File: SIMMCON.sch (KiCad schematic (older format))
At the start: 12 parts, among them U0 PALCE16V8H, U1 74AC(T)245, U2 74AC(T)245

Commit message: update some parts to soic
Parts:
- U1, U2: footprint Housings_DIP:DIP-20_W7.62mm -> Housings_SOIC:SOIC-20W_7.5x12.8mm_Pitch1.27mm
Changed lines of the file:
@@
 F 0 "U1" H 5250 2415 50  0000 C CNN
 F 1 "74AC(T)245" H 5250 2324 50  0000 C CNN
-F 2 "Housings_DIP:DIP-20_W7.62mm" H 5250 1700 50  0001 C CNN
+F 2 "Housings_SOIC:SOIC-20W_7.5x12.8mm_Pitch1.27mm" H 5250 1700 50  0001 C CNN
 F 3 "" H 5250 1700 50  0001 C CNN
 	1    5250 1700
@@
 F 0 "U2" H 5250 3815 50  0000 C CNN
 F 1 "74AC(T)245" H 5250 3724 50  0000 C CNN
-F 2 "Housings_DIP:DIP-20_W7.62mm" H 5250 3100 50  0001 C CNN
+F 2 "Housings_SOIC:SOIC-20W_7.5x12.8mm_Pitch1.27mm" H 5250 3100 50  0001 C CNN
 F 3 "" H 5250 3100 50  0001 C CNN
 	1    5250 3100

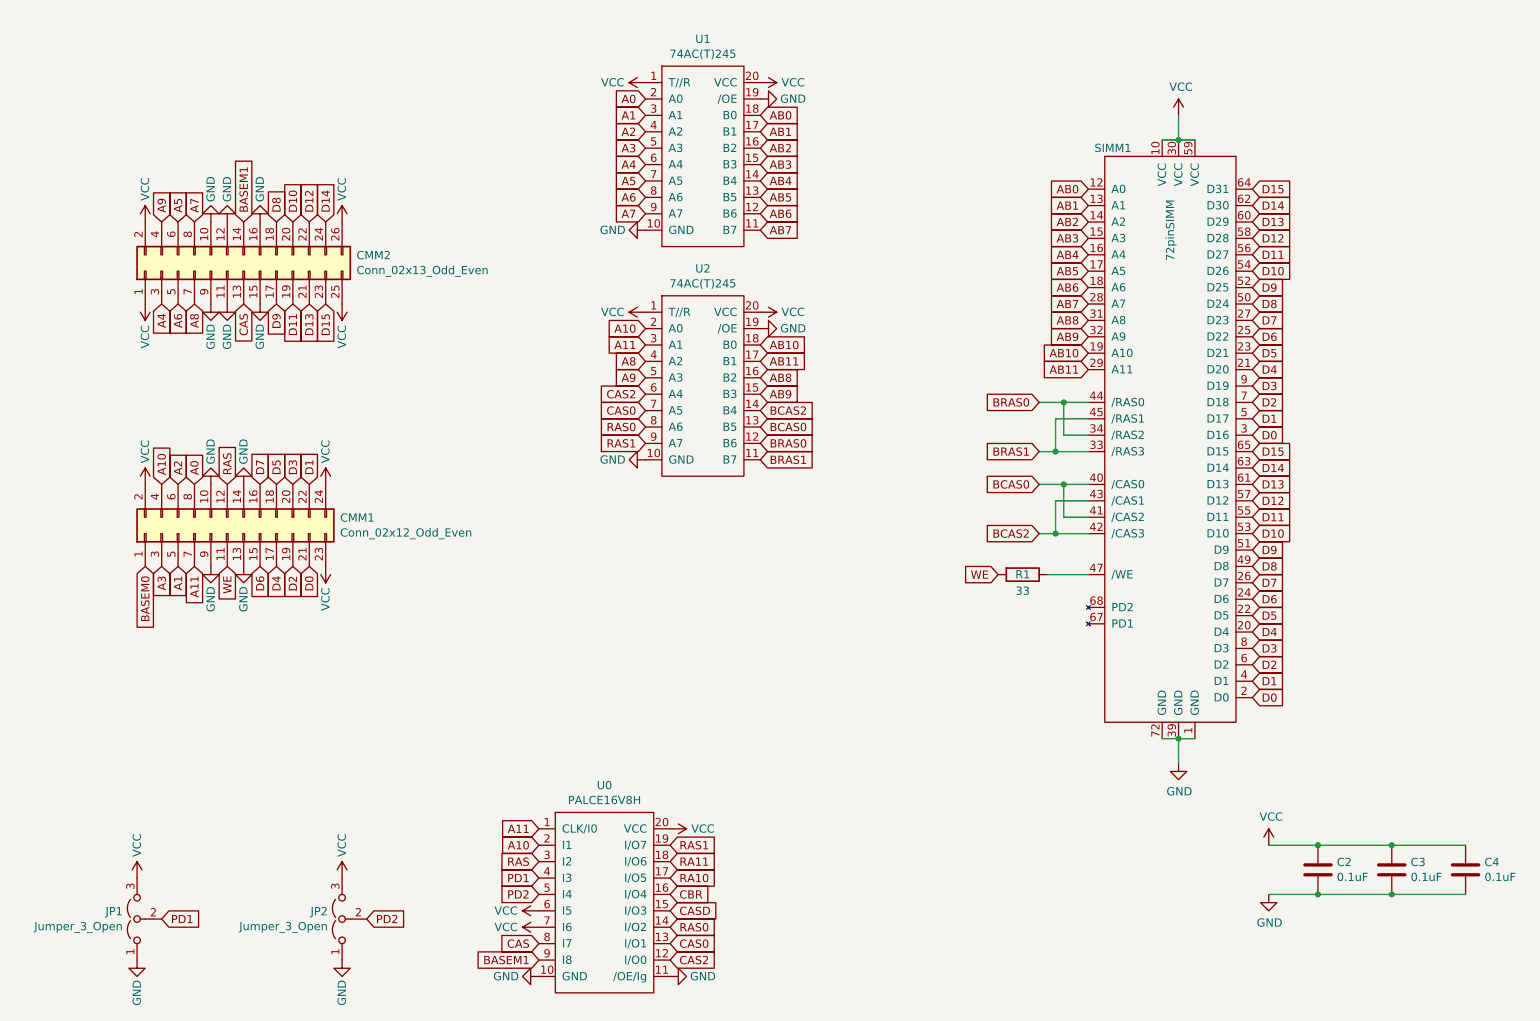
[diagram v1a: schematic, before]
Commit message: updates
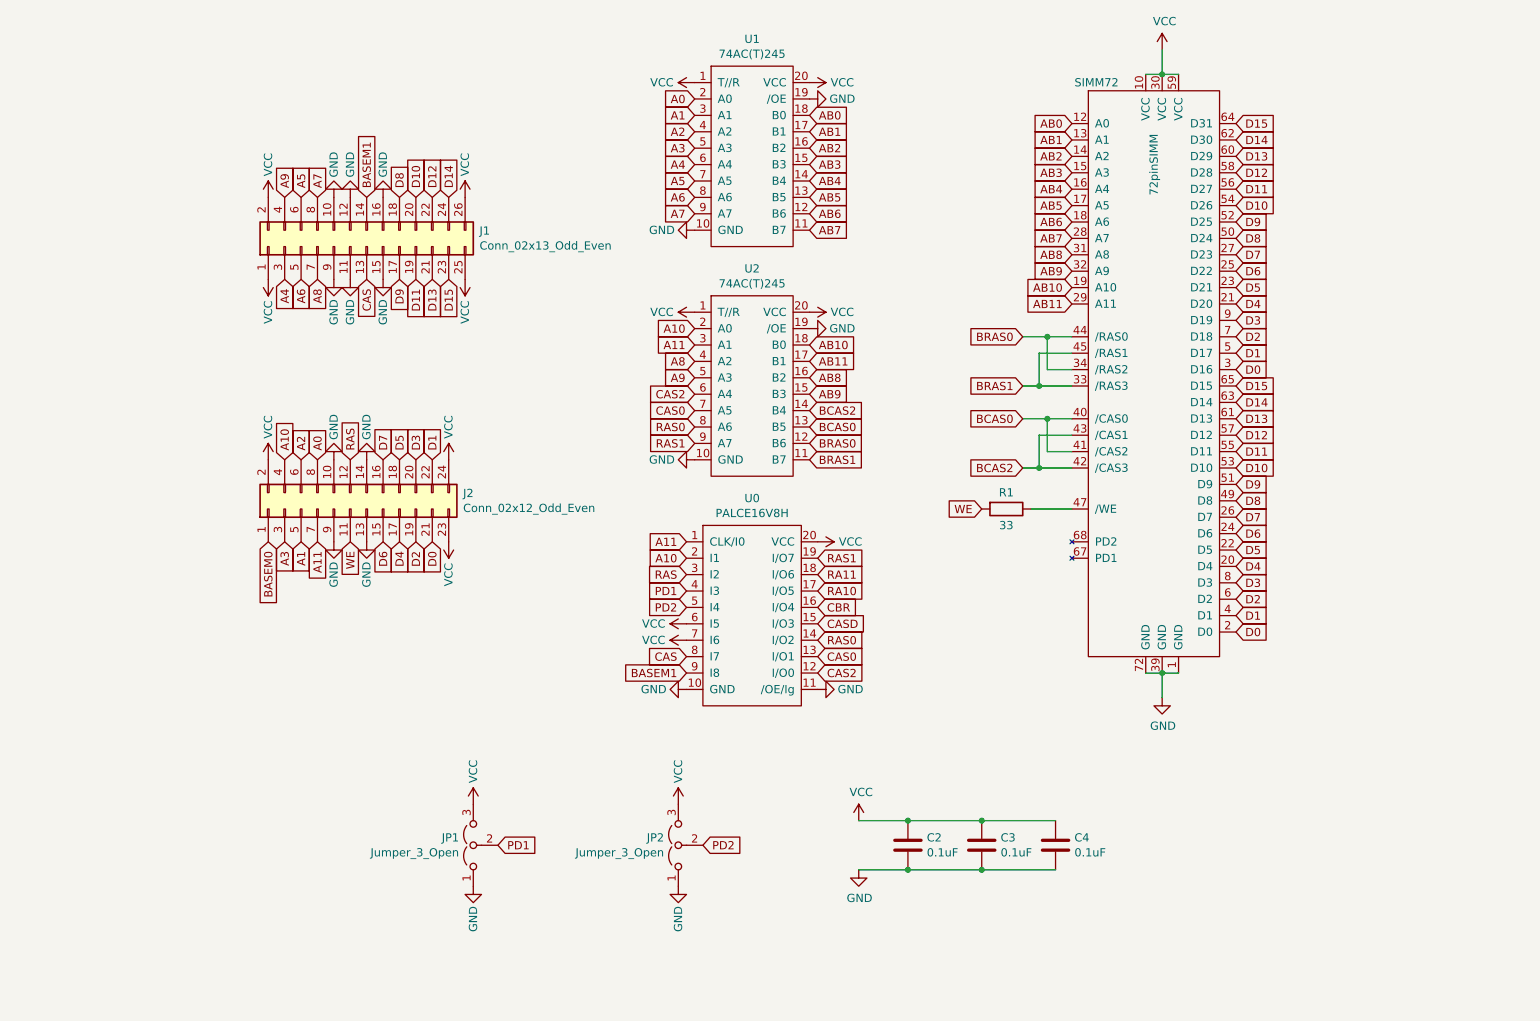
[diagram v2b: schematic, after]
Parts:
- C2, C3, C4: footprint Capacitors_THT:C_Axial_L3.8mm_D2.6mm_P7.50mm_Horizontal -> Capacitors_SMD:C_0805
- R1: footprint Resistors_THT:R_Axial_DIN0204_L3.6mm_D1.6mm_P1.90mm_Vertical -> Resistors_SMD:R_0805
- U0: footprint Housings_DIP:DIP-20_W7.62mm -> Housings_LCC:PLCC-20_SMD-Socket
- renumbered CMM2 to J1, CMM1 to J2, SIMM1 to SIMM72
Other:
- moved on the sheet: C2, C3, C4, J1, J2, JP1, JP2, R1, SIMM72, U0, U1, U2
